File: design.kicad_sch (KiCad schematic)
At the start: 33 parts, among them J1 490107670412, J2 TYPE-C-31-M-12, J4 Conn_02x02_Counter_Clockwise, U1 AP2112K-3.3, U2 TCK107AF,LF, U3 CH340C, U4 TS3USB30RSWR

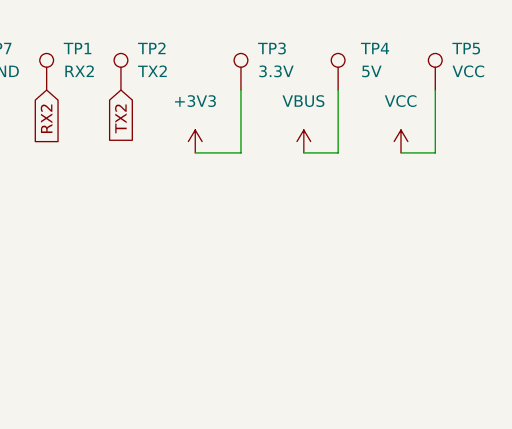
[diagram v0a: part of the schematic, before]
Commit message: update for logo
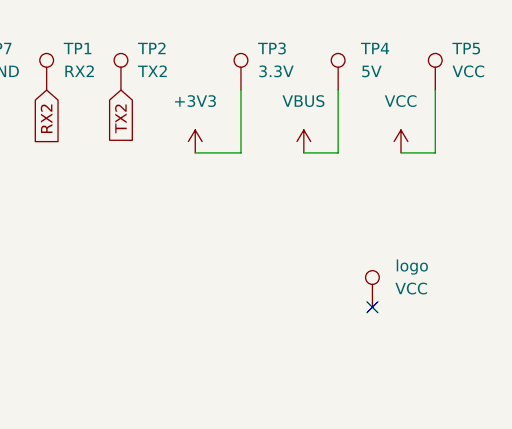
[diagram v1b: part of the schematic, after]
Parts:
- added logo: VCC, TestPoint:TestPoint_Pad_D2.0mm, symbol Connector:TestPoint
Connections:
- no-connect marks 15 -> 16
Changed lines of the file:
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@@
   (no_connect (at 43.815 155.575))
   (no_connect (at 62.865 83.82))
+  (no_connect (at 266.7 154.305))
   (no_connect (at 61.595 155.575))
   (no_connect (at 62.865 96.52))
@@
     (pin "1")
   )
+  (symbol (lib_id "Connector:TestPoint") (at 266.7 154.305 0) (unit 1)
+    (in_bom yes) (on_board yes) (fields_autoplaced)
+    (property "Reference" "logo" (id 0) (at 269.24 149.7329 0)
+      (effects (font (size 1.27 1.27)) (justify left))
+    )
+    (property "Value" "VCC" (id 1) (at 269.24 152.2729 0)
+      (effects (font (size 1.27 1.27)) (justify left))
+    )
+    (property "Footprint" "TestPoint:TestPoint_Pad_D2.0mm" (id 2) (at 271.78 154.305 0)
+      (effects (font (size 1.27 1.27)) hide)
+    )
+    (property "Datasheet" "~" (id 3) (at 271.78 154.305 0)
+      (effects (font (size 1.27 1.27)) hide)
+    )
+    (pin "1")
+  )
   (symbol (lib_id "Device:LED_Small") (at 177.8 26.162 0) (mirror x) (unit 1)
     (in_bom yes) (on_board yes) (fields_autoplaced)
@@
       (reference "U4") (unit 1) (value "TS3USB30RSWR") (footprint "Snapeda:TS3USB30RSWR_QFN40P140X180X55-10N")
     )
+    (path "/30cad120-e725-449e-a695-7e737ec28185"
+      (reference "logo") (unit 1) (value "VCC") (footprint "TestPoint:TestPoint_Pad_D2.0mm")
+    )
   )

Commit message: remove logo
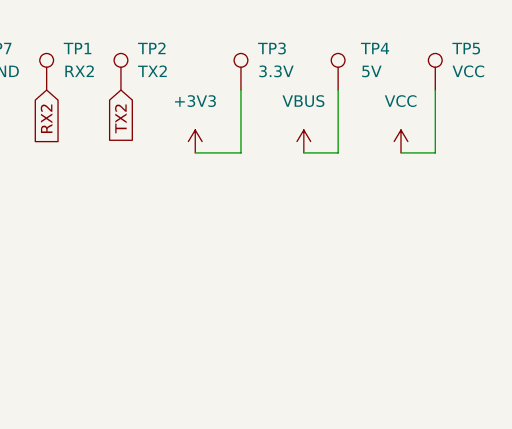
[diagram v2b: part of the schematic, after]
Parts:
- removed logo: VCC, TestPoint:TestPoint_Pad_D2.0mm, symbol Connector:TestPoint
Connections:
- no-connect marks 16 -> 15
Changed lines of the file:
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@@
   (no_connect (at 43.815 155.575))
   (no_connect (at 62.865 83.82))
-  (no_connect (at 266.7 154.305))
   (no_connect (at 61.595 155.575))
   (no_connect (at 62.865 96.52))
@@
     (pin "1")
   )
-  (symbol (lib_id "Connector:TestPoint") (at 266.7 154.305 0) (unit 1)
-    (in_bom yes) (on_board yes) (fields_autoplaced)
-    (property "Reference" "logo" (id 0) (at 269.24 149.7329 0)
-      (effects (font (size 1.27 1.27)) (justify left))
-    )
-    (property "Value" "VCC" (id 1) (at 269.24 152.2729 0)
-      (effects (font (size 1.27 1.27)) (justify left))
-    )
-    (property "Footprint" "TestPoint:TestPoint_Pad_D2.0mm" (id 2) (at 271.78 154.305 0)
-      (effects (font (size 1.27 1.27)) hide)
-    )
-    (property "Datasheet" "~" (id 3) (at 271.78 154.305 0)
-      (effects (font (size 1.27 1.27)) hide)
-    )
-    (pin "1")
-  )
   (symbol (lib_id "Device:LED_Small") (at 177.8 26.162 0) (mirror x) (unit 1)
     (in_bom yes) (on_board yes) (fields_autoplaced)
@@
       (reference "U4") (unit 1) (value "TS3USB30RSWR") (footprint "Snapeda:TS3USB30RSWR_QFN40P140X180X55-10N")
     )
-    (path "/30cad120-e725-449e-a695-7e737ec28185"
-      (reference "logo") (unit 1) (value "VCC") (footprint "TestPoint:TestPoint_Pad_D2.0mm")
-    )
   )
